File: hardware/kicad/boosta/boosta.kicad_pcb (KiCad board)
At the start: 2 copper layers, 100.9 x 90.4 mm, 2 parts, among them J1 Conn_01x08_Female, J2 Screw_Terminal_01x02

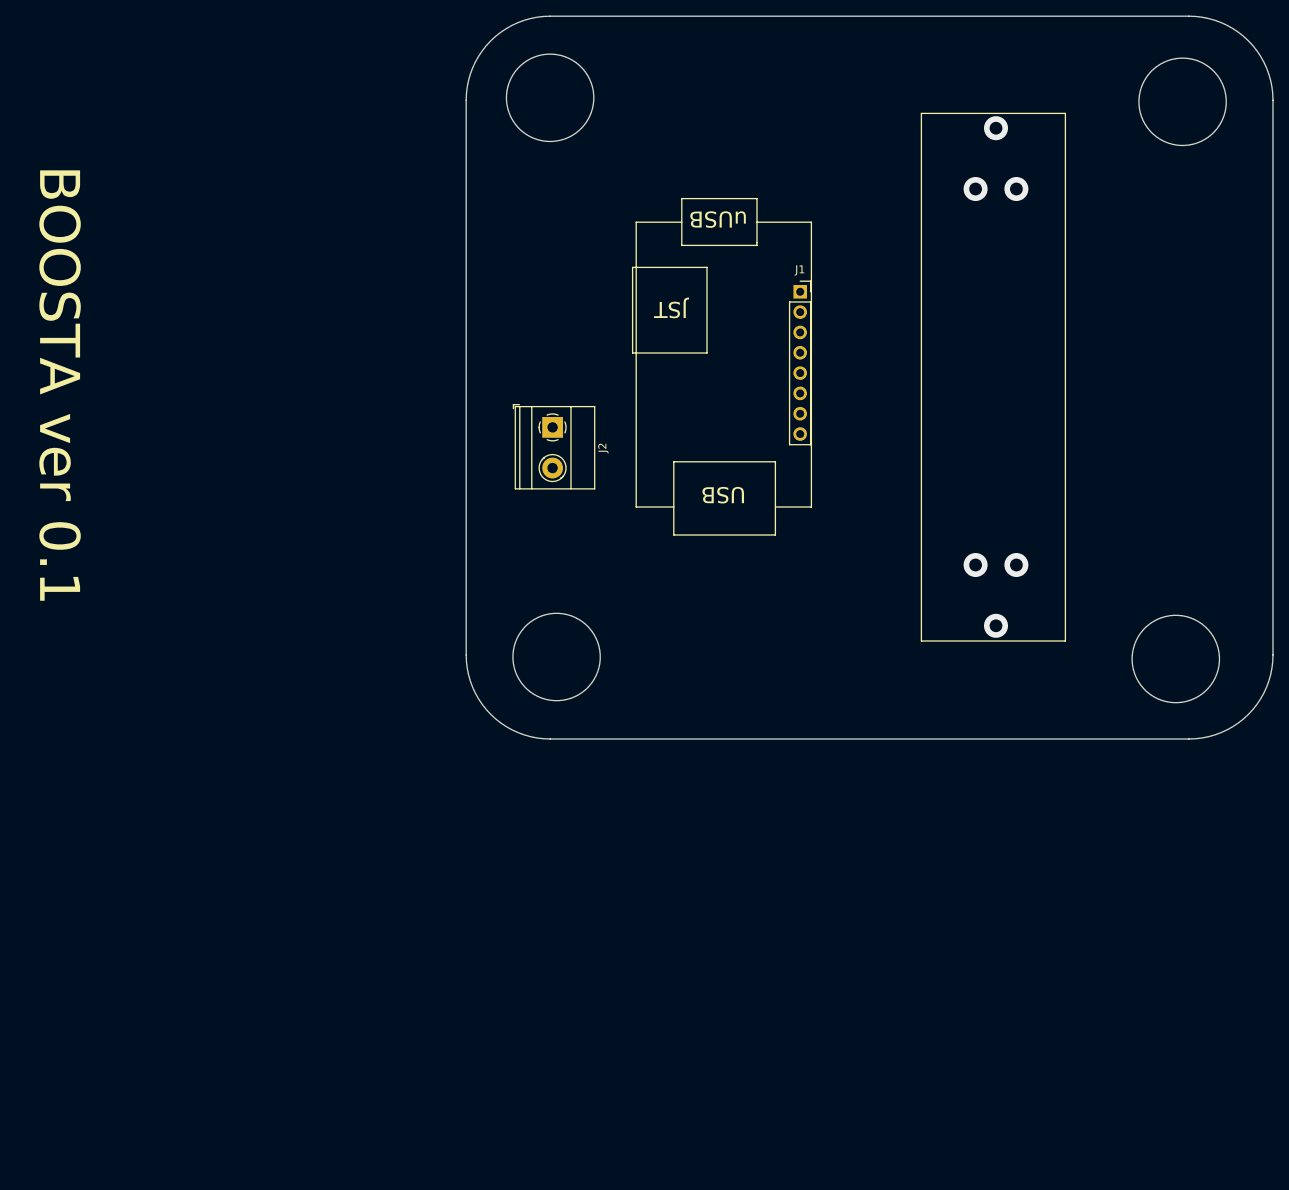
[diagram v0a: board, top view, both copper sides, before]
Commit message: update
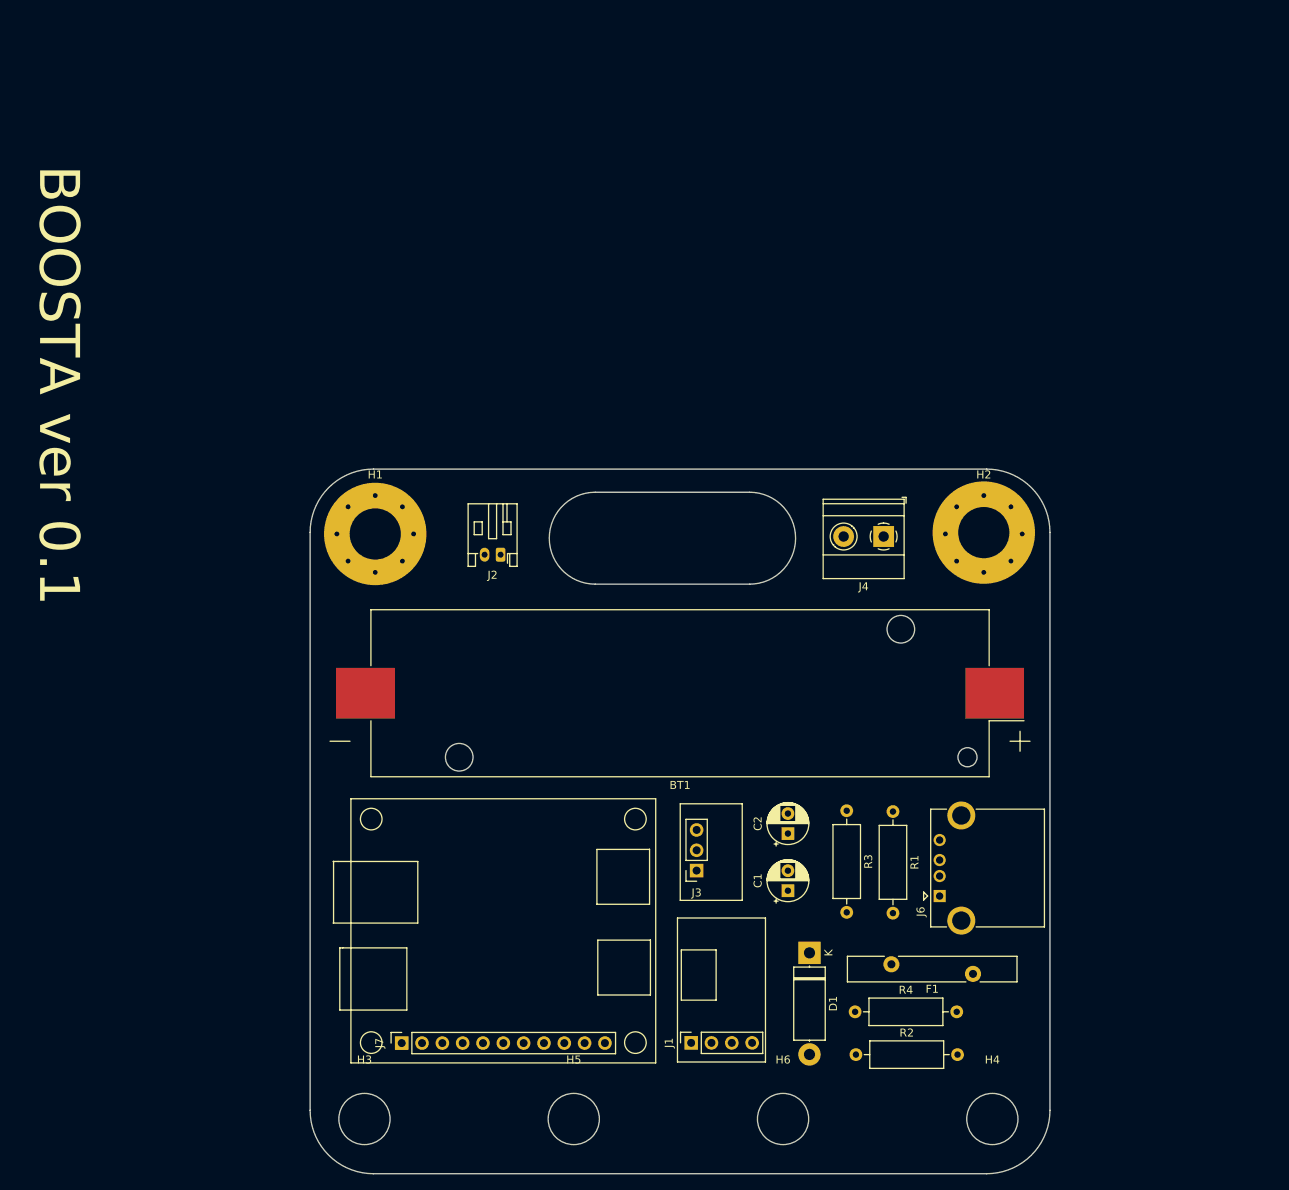
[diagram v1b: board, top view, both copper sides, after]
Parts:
- added BT1: Battery_Cell, Battery:BatteryHolder_Keystone_1042_1x18650, F.Cu at (76.5, 105.5)
- added C1: 10uF, Capacitor_THT:CP_Radial_D5.0mm_P2.50mm, F.Cu at (90.0, 130.2)
- added C2: 22uF, Capacitor_THT:CP_Radial_D5.0mm_P2.50mm, F.Cu at (90.0, 123.1)
- added D1: D, Diode_THT:D_5W_P12.70mm_Horizontal, F.Cu at (92.7, 138.0)
- added F1: Polyfuse, Fuse:Fuse_Bourns_MF-RHT1100, F.Cu at (113.2, 140.6)
- added H1: MountingHole_Pad, MountingHole:MountingHole_6.4mm_M6_Pad_Via, F.Cu at (38.4, 85.6)
- added H2: MountingHole_Pad, MountingHole:MountingHole_6.4mm_M6_Pad_Via, F.Cu at (114.5, 85.6)
- added H3: MountingHole, MountingHole:MountingHole_6.4mm_M6, F.Cu at (37.1, 158.8)
- added H4: MountingHole, MountingHole:MountingHole_6.4mm_M6, F.Cu at (115.6, 158.8)
- added H5: MountingHole, MountingHole:MountingHole_6.4mm_M6, F.Cu at (63.2, 158.8)
- added H6: MountingHole, MountingHole:MountingHole_6.4mm_M6, F.Cu at (89.4, 158.8)
- added J3: Conn_01x03_Female, Connector_PinSocket_2.54mm:PinSocket_1x03_P2.54mm_Vertical, F.Cu at (78.6, 127.7)
- added J4: Conn_01x02_Female, TerminalBlock_Phoenix:TerminalBlock_Phoenix_MKDS-1,5-2_1x02_P5.00mm_Horizontal, F.Cu at (102.0, 85.9)
- added J6: USB_A, Connector_USB:USB_A_CONNFLY_DS1095-WNR0, F.Cu at (109.0, 130.9)
- added J7: Conn_01x11_Female, Connector_PinSocket_2.54mm:PinSocket_1x11_P2.54mm_Vertical, F.Cu at (41.7, 149.3)
- added R1: 75K, Resistor_THT:R_Axial_DIN0309_L9.0mm_D3.2mm_P12.70mm_Horizontal, F.Cu at (103.1, 120.3)
- added R2: 49.9K, Resistor_THT:R_Axial_DIN0309_L9.0mm_D3.2mm_P12.70mm_Horizontal, F.Cu at (98.5, 150.7)
- added R3: 75K, Resistor_THT:R_Axial_DIN0309_L9.0mm_D3.2mm_P12.70mm_Horizontal, F.Cu at (97.4, 120.2)
- added R4: 49.9K, Resistor_THT:R_Axial_DIN0309_L9.0mm_D3.2mm_P12.70mm_Horizontal, F.Cu at (98.4, 145.4)
- J1: value Conn_01x08_Female -> Conn_01x04_Female; footprint Connector_PinSocket_2.54mm:PinSocket_1x08_P2.54mm_Vertical -> Connector_PinSocket_2.54mm:PinSocket_1x04_P2.54mm_Vertical
- J2: value Screw_Terminal_01x02 -> Conn_01x02_Female; footprint TerminalBlock_Phoenix:TerminalBlock_Phoenix_MKDS-1,5-2-5.08_1x02_P5.08mm_Horizontal -> Connector_JST:JST_PH_S2B-PH-K_1x02_P2.00mm_Horizontal
- moved J1 94.9 mm to (77.9, 149.2), turned to 90 degrees
- moved J2 17.2 mm to (54.1, 88.2), turned to 180 degrees
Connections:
- J1 pad 1: 5V -> OUT
- J1 pad 3: (no net) -> 5VBOOST
- J1 pad 4: GND -> (no net)
- J2 pad 1: GND -> (no net)
- J2 pad 2: 5V -> (no net)
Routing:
- net (no net): vias 6 -> 0
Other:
- board size 100.9 x 90.4 mm -> 92.5 x 88.1 mm
- board text removed: "JST"
- board text removed: "USB"
- board text removed: "uUSB"
